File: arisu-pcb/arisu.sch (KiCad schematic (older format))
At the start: 40 parts, among them J1 USB_B_Micro, J10 PF6, J11 PF7, J12 VCC, J13 D+, J14 D-, J15 GND, J2 MISO, J3 VCC, J4 SCK, J5 MOSI, J6 RES, J7 GND, J8 PF4, J9 PF5, U1 USBLC6-2SC6, U3 AT90USB1286-MU, Y1 Crystal_GND24

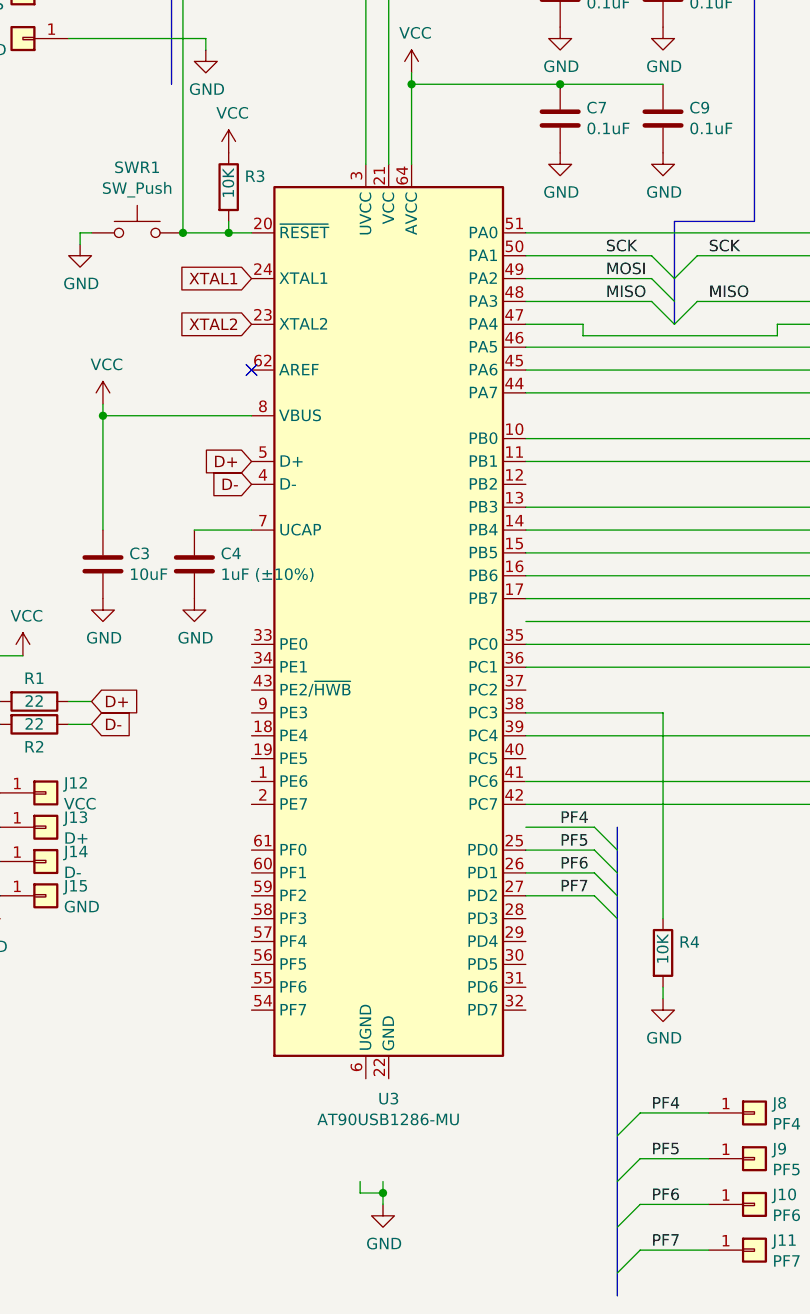
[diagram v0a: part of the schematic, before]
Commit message: cap nhat 18:16 27/2/2021
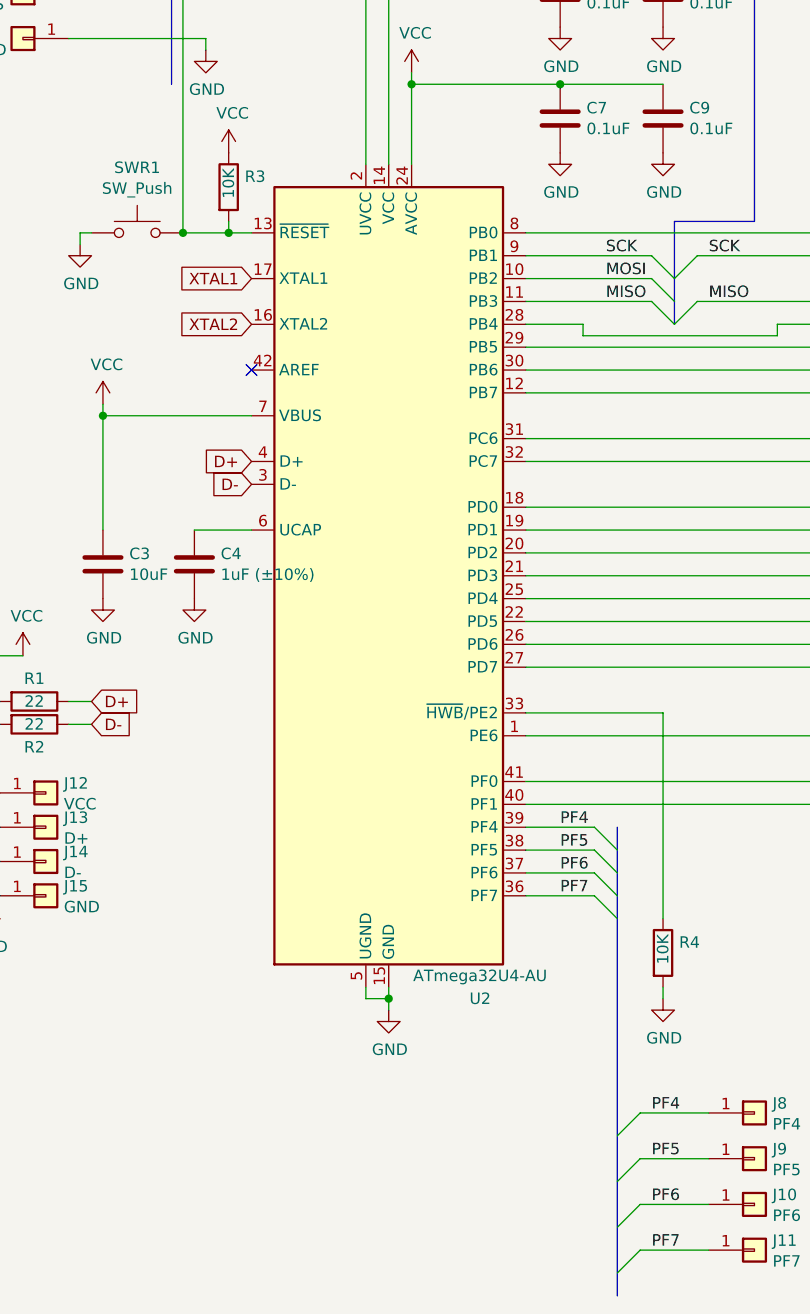
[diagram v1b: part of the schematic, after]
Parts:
- removed U3: AT90USB1286-MU, Package_DFN_QFN:QFN-64-1EP_9x9mm_P0.5mm_EP7.5x7.5mm, symbol MCU_Microchip_AVR:AT90USB1286-MU
- added U2: ATmega32U4-AU, Housings_QFP:TQFP-44_10x10mm_Pitch0.8mm, symbol MCU_Microchip_ATmega:ATmega32U4-AU
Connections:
- net D+: now also U2.4 (D+)
- net D-: now also U2.3 (D-)
- net GND: now also U2.15 (GND), U2.23 (GND), U2.35 (GND), U2.43 (GND), U2.5 (UGND)
- net MISO: now also U2.11 (PB3)
- net MOSI: now also U2.10 (PB2)
- net PF4: now also U2.39 (PF4)
- net PF5: now also U2.38 (PF5)
- net PF6: now also U2.37 (PF6)
- net PF7: now also U2.36 (PF7)
- net SCK: now also U2.9 (PB1)
- net VCC: now also U2.14 (VCC), U2.2 (UVCC), U2.24 (AVCC), U2.34 (VCC), U2.44 (AVCC), U2.7 (VBUS)
- net XTAL1: now also U2.17 (XTAL1)
- net XTAL2: now also U2.16 (XTAL2)
- net col0: now also U2.41 (PF0)
- net col1: now also U2.40 (PF1)
- net col10: now also U2.29 (PB5)
- net col11: now also U2.28 (PB4)
- net col12: now also U2.27 (PD7)
- net col13: now also U2.26 (PD6)
- net col2: now also U2.1 (PE6)
- net col3: now also U2.32 (PC7)
- net col4: now also U2.31 (PC6)
- net col5: now also U2.30 (PB6)
- net col6: now also U2.25 (PD4)
- net col8: now also U2.8 (PB0)
- net col9: now also U2.12 (PB7)
- net row0: now also U2.18 (PD0)
- net row1: now also U2.19 (PD1)
- net row2: now also U2.20 (PD2)
- net row3: now also U2.21 (PD3)
- net row4: now also U2.22 (PD5)
- net ~RES~: now also U2.13 (~RESET)
- net at C4.1: now also U2.6 (UCAP)
- net at R4.1: now also U2.33 (~HWB~/PE2)
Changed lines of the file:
@@
 $EndDescr
+$Comp
+L MCU_Microchip_ATmega:ATmega32U4-AU U2
+U 1 1 5C4B1F82
+P 4500 4250
+F 0 "U2" H 4900 2400 50  0000 C CNN
+F 1 "ATmega32U4-AU" H 4900 2500 50  0000 C CNN
+F 2 "Housings_QFP:TQFP-44_10x10mm_Pitch0.8mm" H 4500 4250 50  0001 C CIN
+F 3 "http://ww1.microchip.com/downloads/en/DeviceDoc/Atmel-7766-8-bit-AVR-ATmega16U4-32U4_Datasheet.pdf" H 4500 4250 50  0001 C CNN
+	1    4500 4250
+	1    0    0    -1
+$EndComp
 $Comp
 L Connector:USB_B_Micro J1
@@
 L power:GND #PWR0116
 U 1 1 5C4F0424
-P 4475 7000
-F 0 "#PWR0116" H 4475 6750 50  0001 C CNN
-F 1 "GND" H 4480 6827 50  0000 C CNN
-F 2 "" H 4475 7000 50  0001 C CNN
-F 3 "" H 4475 7000 50  0001 C CNN
-	1    4475 7000
-	1    0    0    -1
-$EndComp
-Wire Wire Line
-	4375 6900 4375 6950
-Wire Wire Line
-	4375 6950 4475 6950
-Wire Wire Line
-	4475 6950 4475 7000
-Wire Wire Line
-	4475 6900 4475 6950
-Connection ~ 4475 6950
+P 4500 6150
+F 0 "#PWR0116" H 4500 5900 50  0001 C CNN
+F 1 "GND" H 4505 5977 50  0000 C CNN
+F 2 "" H 4500 6150 50  0001 C CNN
+F 3 "" H 4500 6150 50  0001 C CNN
+	1    4500 6150
+	1    0    0    -1
+$EndComp
+Wire Wire Line
+	4400 6050 4400 6100
+Wire Wire Line
+	4400 6100 4500 6100
+Wire Wire Line
+	4500 6100 4500 6150
+Wire Wire Line
+	4500 6050 4500 6100
+Connection ~ 4500 6100
 $Comp
 L power:VCC #PWR0117
@@
 Wire Wire Line
 	1900 4600 2750 4600
-$Comp
-L MCU_Microchip_AVR:AT90USB1286-MU U3
-U 1 1 6013B83C
-P 4500 4450
-F 0 "U3" H 4500 2361 50  0000 C CNN
-F 1 "AT90USB1286-MU" H 4500 2270 50  0000 C CNN
-F 2 "Package_DFN_QFN:QFN-64-1EP_9x9mm_P0.5mm_EP7.5x7.5mm" H 4500 4450 50  0001 C CIN
-F 3 "http://ww1.microchip.com/downloads/en/DeviceDoc/doc7593.pdf" H 4500 4450 50  0001 C CNN
-	1    4500 4450
-	1    0    0    -1
-$EndComp
 Wire Bus Line
 	5750 2700 5750 3150
